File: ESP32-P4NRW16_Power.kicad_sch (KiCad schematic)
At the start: 32 parts, among them U1 ESP32-P4NRW16

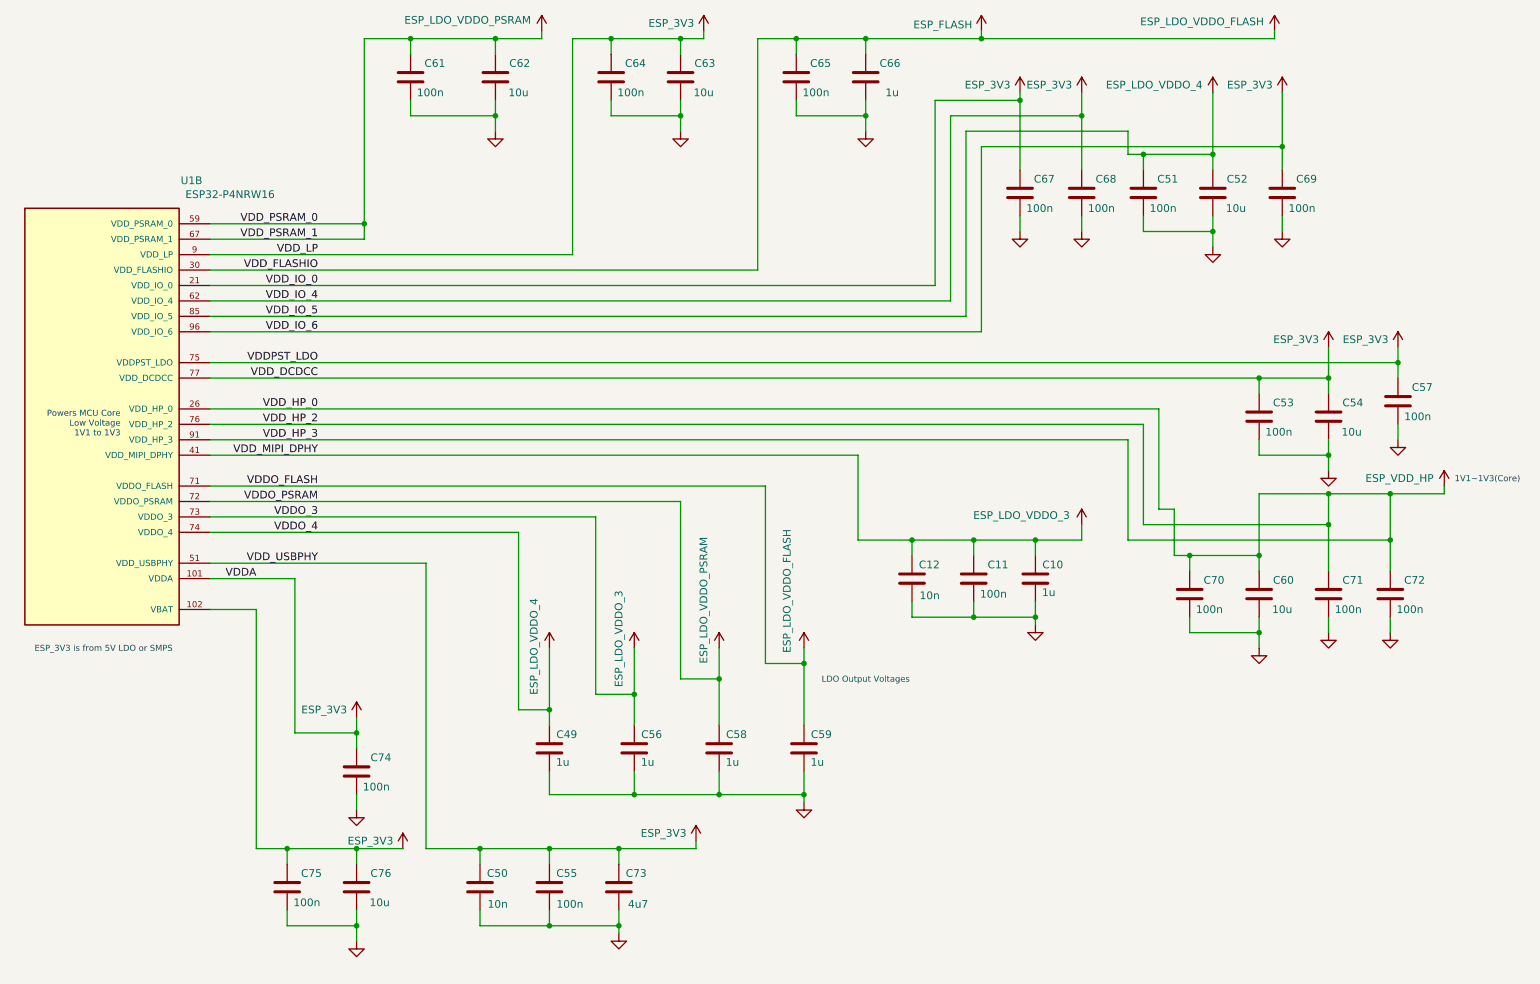
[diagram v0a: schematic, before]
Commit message: VDD_HP_1 Update
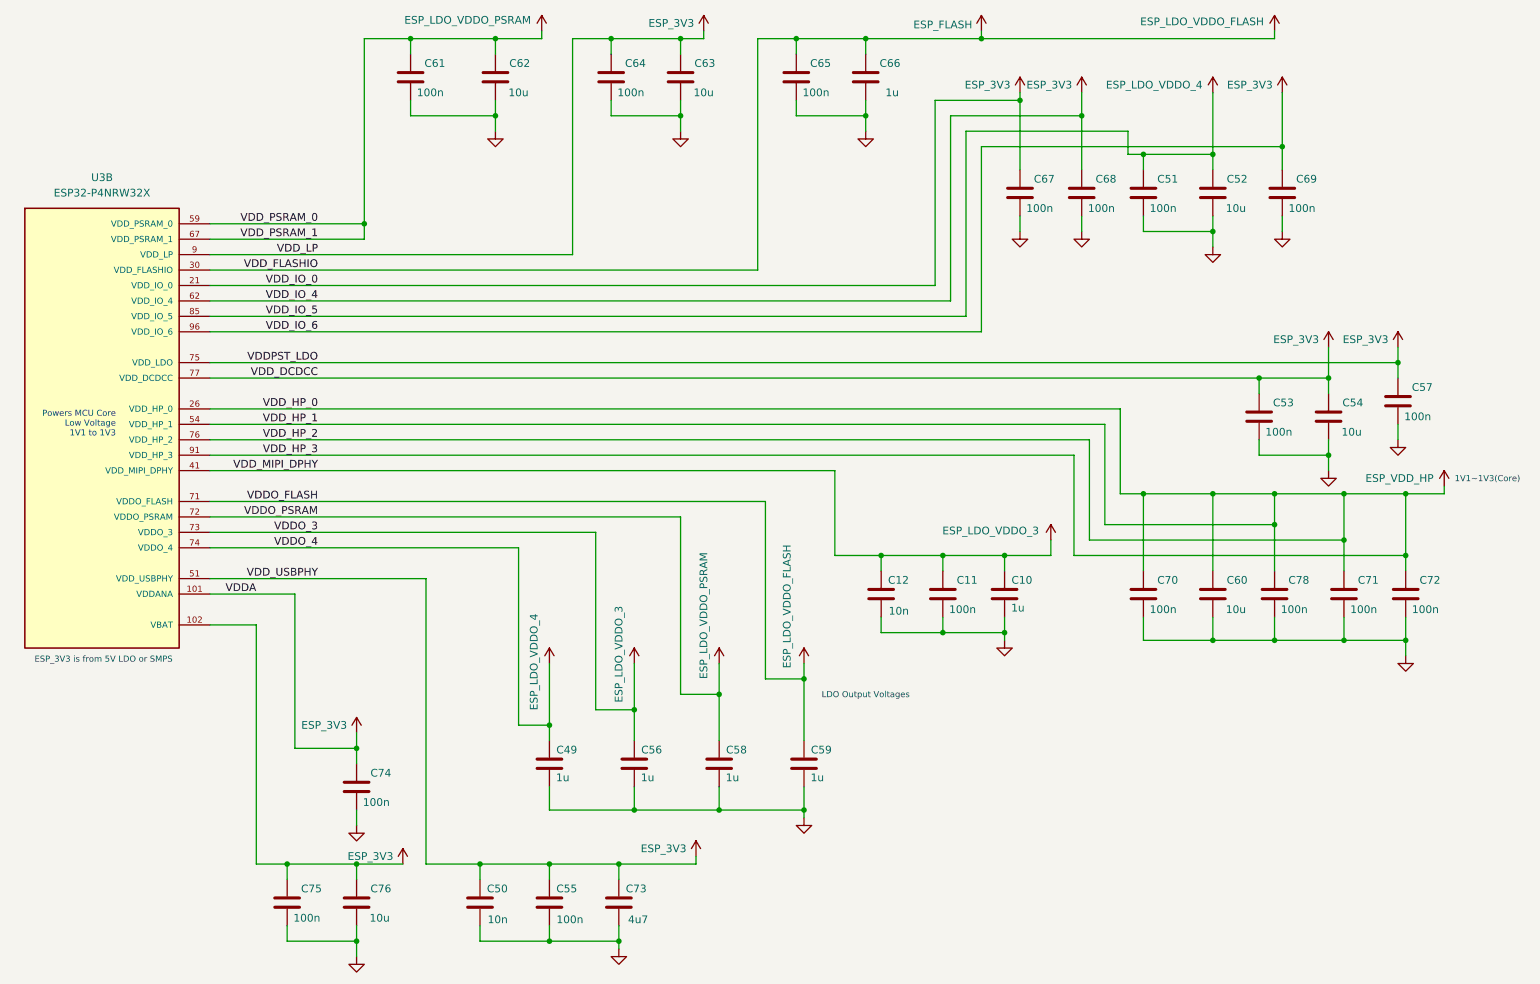
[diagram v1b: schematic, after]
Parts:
- removed U1: ESP32-P4NRW16, Personal_Project:ESP32-P4NRW16, symbol Personal_Projects:ESP32-P4NRW16
- added C78: 100n, Capacitor_SMD:C_0603_1608Metric, symbol Device:C
- added U3: ESP32-P4NRW32X, Personal_Project:ESP32-P4NRW16, symbol Personal_Components:ESP32-P4NRW32X
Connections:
- net ESP_3V3: now also U3.101 (VDDANA), U3.102 (VBAT), U3.21 (VDD_IO_0), U3.51 (VDD_USBPHY), U3.62 (VDD_IO_4), U3.75 (VDD_LDO), U3.77 (VDD_DCDCC), U3.9 (VDD_LP), U3.96 (VDD_IO_6)
- net ESP_FLASH: now also U3.30 (VDD_FLASHIO), U3.71 (VDDO_FLASH)
- net ESP_LDO_VDDO_3: now also U3.41 (VDD_MIPI_DPHY), U3.73 (VDDO_3)
- net ESP_LDO_VDDO_4: now also U3.74 (VDDO_4), U3.85 (VDD_IO_5)
- net ESP_LDO_VDDO_PSRAM: now also U3.59 (VDD_PSRAM_0), U3.67 (VDD_PSRAM_1), U3.72 (VDDO_PSRAM)
- net ESP_VDD_HP: now also C78.1, U3.26 (VDD_HP_0), U3.54 (VDD_HP_1), U3.76 (VDD_HP_2), U3.91 (VDD_HP_3)
- net GND: now also C78.2
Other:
- moved on the sheet: C10, C11, C12, C49, C50, C55, C56, C58, C59, C60, C70, C71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

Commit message: PCB Layout Update
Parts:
- C52, C54: footprint Capacitor_SMD:C_1206_3216Metric -> Capacitor_SMD:C_0805_2012Metric
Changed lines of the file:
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@@
 			)
 		)
-		(property "Footprint" "Capacitor_SMD:C_1206_3216Metric"
+		(property "Footprint" "Capacitor_SMD:C_0805_2012Metric"
 			(at 247.9548 93.98 0)
 			(hide yes)
@@
 			)
 		)
-		(property "Footprint" "Capacitor_SMD:C_1206_3216Metric"
+		(property "Footprint" "Capacitor_SMD:C_0805_2012Metric"
 			(at 228.9048 57.15 0)
 			(hide yes)

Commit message: RF_Layout
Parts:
- C76: footprint Capacitor_SMD:C_1206_3216Metric -> Capacitor_SMD:C_0805_2012Metric
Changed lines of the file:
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@@
 			)
 		)
-		(property "Footprint" "Capacitor_SMD:C_1206_3216Metric"
+		(property "Footprint" "Capacitor_SMD:C_0805_2012Metric"
 			(at 87.9348 173.99 0)
 			(hide yes)
